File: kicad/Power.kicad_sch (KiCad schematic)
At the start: 20 parts, among them IC1 AP2112K-3.3TRG1, IC2 ADP1713AUJZ-3.3-R7, J3 Conn_BATT, U3 TP4056-42-ESOP8

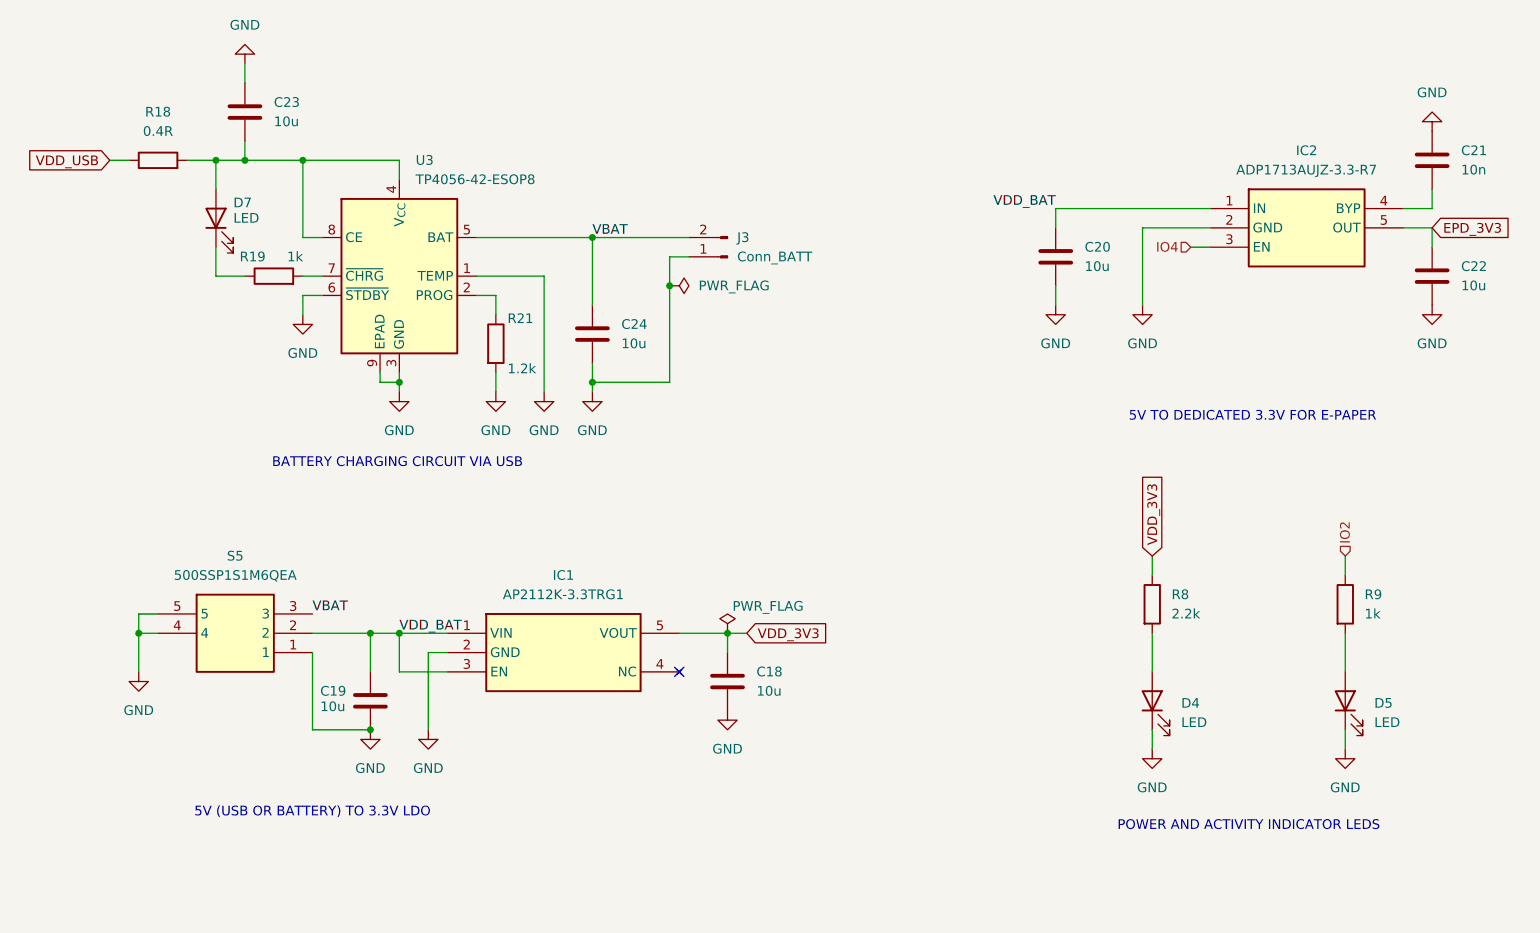
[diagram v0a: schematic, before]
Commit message: updating chinese chips
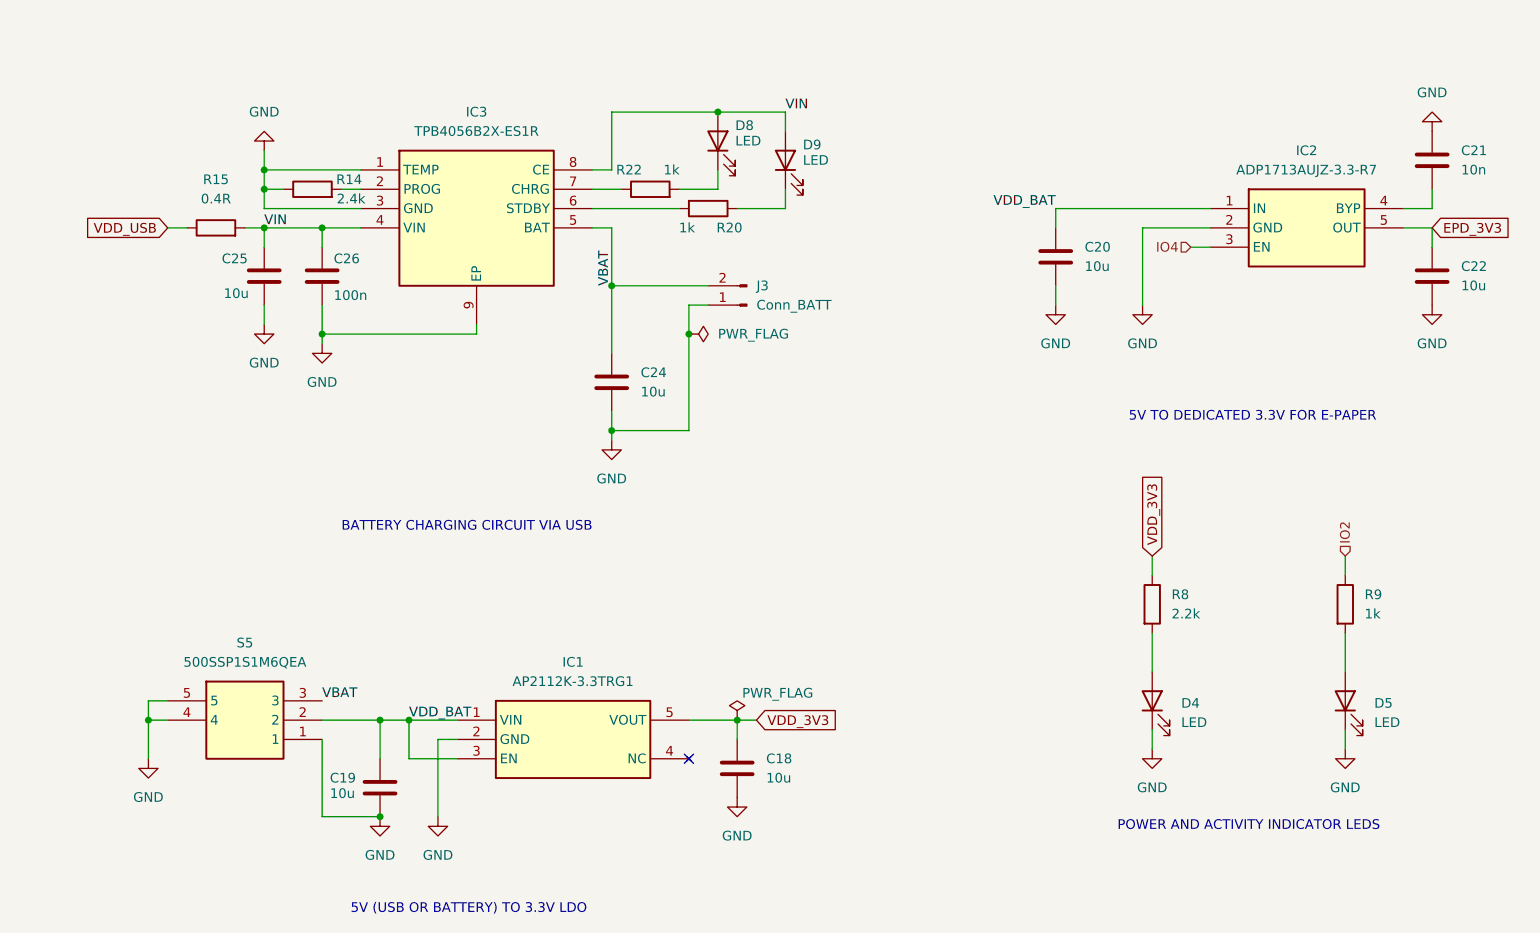
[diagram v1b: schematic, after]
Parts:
- removed C23: 10u, Capacitor_SMD:C_0603_1608Metric_Pad1.08x0.95mm_HandSolder, symbol Device:C
- removed D7: LED, LED_SMD:LED_0805_2012Metric_Pad1.15x1.40mm_HandSolder, symbol Device:LED
- removed R18: 0.4R, Resistor_SMD:R_1206_3216Metric_Pad1.30x1.75mm_HandSolder, symbol Device:R
- removed R19: 1k, Resistor_SMD:R_0603_1608Metric_Pad0.98x0.95mm_HandSolder, symbol Device:R
- removed R21: 1.2k, Resistor_SMD:R_0603_1608Metric_Pad0.98x0.95mm_HandSolder, symbol Device:R
- removed U3: TP4056-42-ESOP8, Package_SO:SOIC-8-1EP_3.9x4.9mm_P1.27mm_EP2.41x3.3mm_ThermalVias, symbol Battery_Management:TP4056-42-ESOP8
- added C25: 10u, Capacitor_SMD:C_0603_1608Metric_Pad1.08x0.95mm_HandSolder, symbol Device:C
- added C26: 100n, Capacitor_SMD:C_0603_1608Metric_Pad1.08x0.95mm_HandSolder, symbol Device:C
- added D8, D9: LED, LED_SMD:LED_0805_2012Metric_Pad1.15x1.40mm_HandSolder, symbol Device:LED
- added IC3: TPB4056B2X-ES1R, e-reader:TPB4056B2X-ES1R, symbol e-reader:TPB4056B2X-ES1R
- added R14: 2.4k, e-reader:TPB4056B2X-ES1R, symbol Device:R
- added R15: 0.4R, Resistor_SMD:R_1206_3216Metric_Pad1.30x1.75mm_HandSolder, symbol Device:R
- added R20, R22: 1k, Resistor_SMD:R_0603_1608Metric_Pad0.98x0.95mm_HandSolder, symbol Device:R
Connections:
- net GND: now also C25.2, C26.2, IC3.1 (TEMP), IC3.3 (GND), IC3.9 (EP), R14.1
- net VBAT: now also IC3.5 (BAT)
- net VDD_USB: now also R15.1
- new net: IC3.7 (CHRG), R22.1
- new net: D8.1 (K), R22.2
- new net: D9.1 (K), R20.1
- new net: IC3.2 (PROG), R14.2
- new net: IC3.6 (STDBY), R20.2
- new net VIN: C25.1, C26.1, D8.2 (A), D9.2 (A), IC3.4 (VIN), IC3.8 (CE), R15.2
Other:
- moved on the sheet: C18, C19, C24, IC1, J3, S5
